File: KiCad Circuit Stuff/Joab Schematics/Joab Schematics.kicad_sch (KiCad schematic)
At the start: 60 parts, among them J1 Conn_02x16_Odd_Even, J2 Conn_01x02, U1 MT3608, U2 AMS1117-3.3, U3 TP4056, U4 INA219AIDCNR, U6 TS5A3159DCKR, U7 TPS5430DDAR

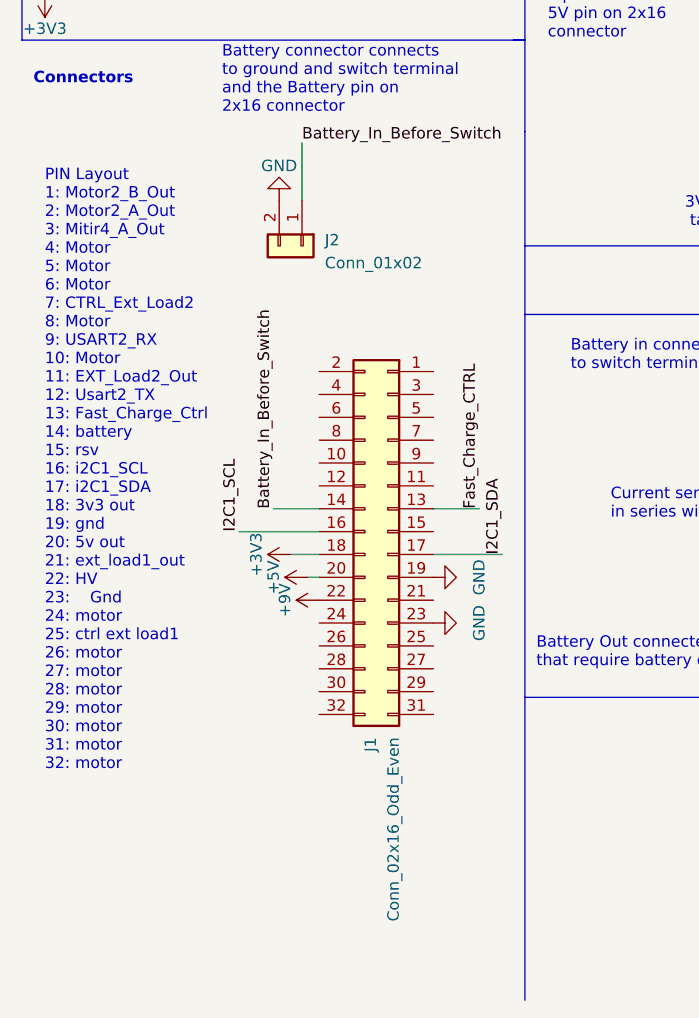
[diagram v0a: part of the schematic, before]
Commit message: Added ReadMe and other minor changes
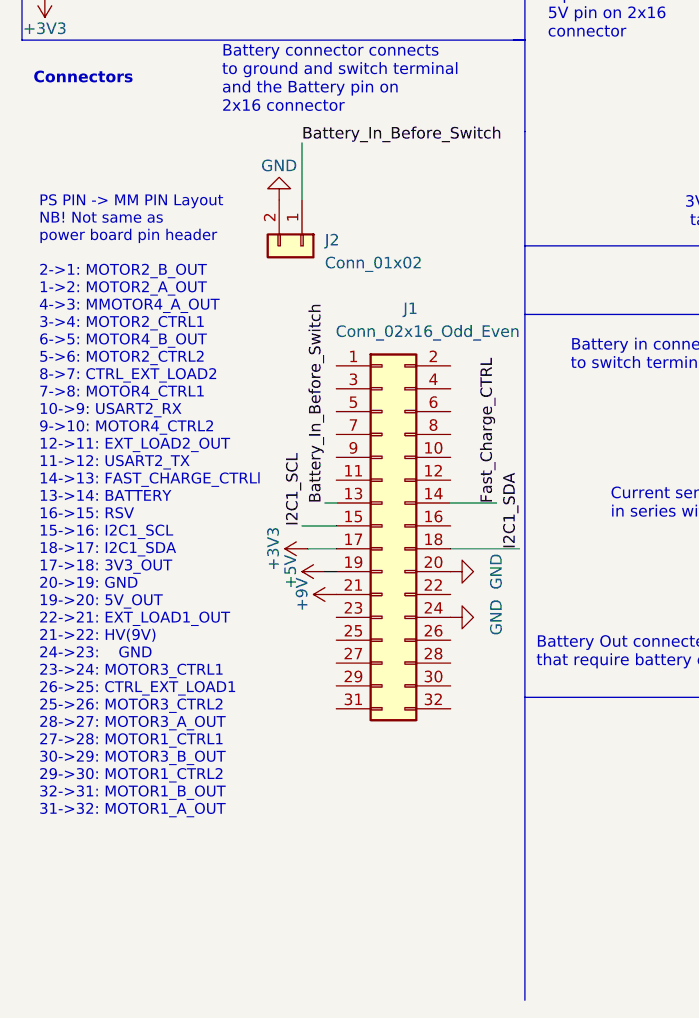
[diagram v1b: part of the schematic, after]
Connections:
- net +3V3: now also J1.17 (Pin_17); no longer J1.18 (Pin_18)
- net +5V: now also J1.19 (Pin_19); no longer J1.20 (Pin_20)
- net +9V: now also J1.21 (Pin_21); no longer J1.22 (Pin_22)
- net Battery_In_Before_Switch: now also J1.13 (Pin_13); no longer J1.14 (Pin_14)
- net Fast_Charge_CTRL: now also J1.14 (Pin_14); no longer J1.13 (Pin_13)
- net GND: now also J1.20 (Pin_20), J1.24 (Pin_24); no longer J1.19 (Pin_19), J1.23 (Pin_23)
- net I2C1_SCL: now also J1.15 (Pin_15); no longer J1.16 (Pin_16)
- net I2C1_SDA: now also J1.18 (Pin_18); no longer J1.17 (Pin_17)
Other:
- note added: "PS PIN -> MM PIN Layout NB! Not same as power board pin header 2->1: MOTOR2_B_OUT 1->2: MOTOR2_A_OUT 4->3: MMOTOR4_A_OUT 3->4: MOTOR2_CTRL1 6->5: MOTOR4_B_OUT 5->6: MOTOR2_CTRL2 8->7: CTRL_EXT_LOAD2 7->8: MOTOR4_CTRL1 10->9: USART2_RX 9->10: MOTOR4_CTRL2 12->11: EXT_LOAD2_OUT 11->12: USART2_TX 14->13: FAST_CHARGE_CTRLl 13->14: BATTERY 16->15: RSV 15->16: I2C1_SCL 18->17: I2C1_SDA 17->18: 3V3_OUT 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"
- note removed: "PIN Layout 1: Motor2_B_Out 2: Motor2_A_Out 3: Mitir4_A_Out 4: Motor 5: Motor 6: Motor 7: CTRL_Ext_Load2 8: Motor 9: USART2_RX 10: Motor 11: EXT_Load2_Out 12: Usart2_TX 13: Fast_Charge_Ctrl 14: battery 15: rsv 16: i2C1_SCL 17: i2C1_SDA 18: 3v3 out 19: gnd 20: 5v out 21: ext_load1_out 22: HV 23: Gnd 24: motor 25: ctrl ext load1 26: motor 27: motor 28: motor 29: motor 30: motor 31: motor 32: motor"
- moved on the sheet: J1
